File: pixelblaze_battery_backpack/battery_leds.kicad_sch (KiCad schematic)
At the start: 23 parts, among them J10 Conn_01x04, J11 Conn_01x04, J14 Conn_01x04, J15 Conn_01x04

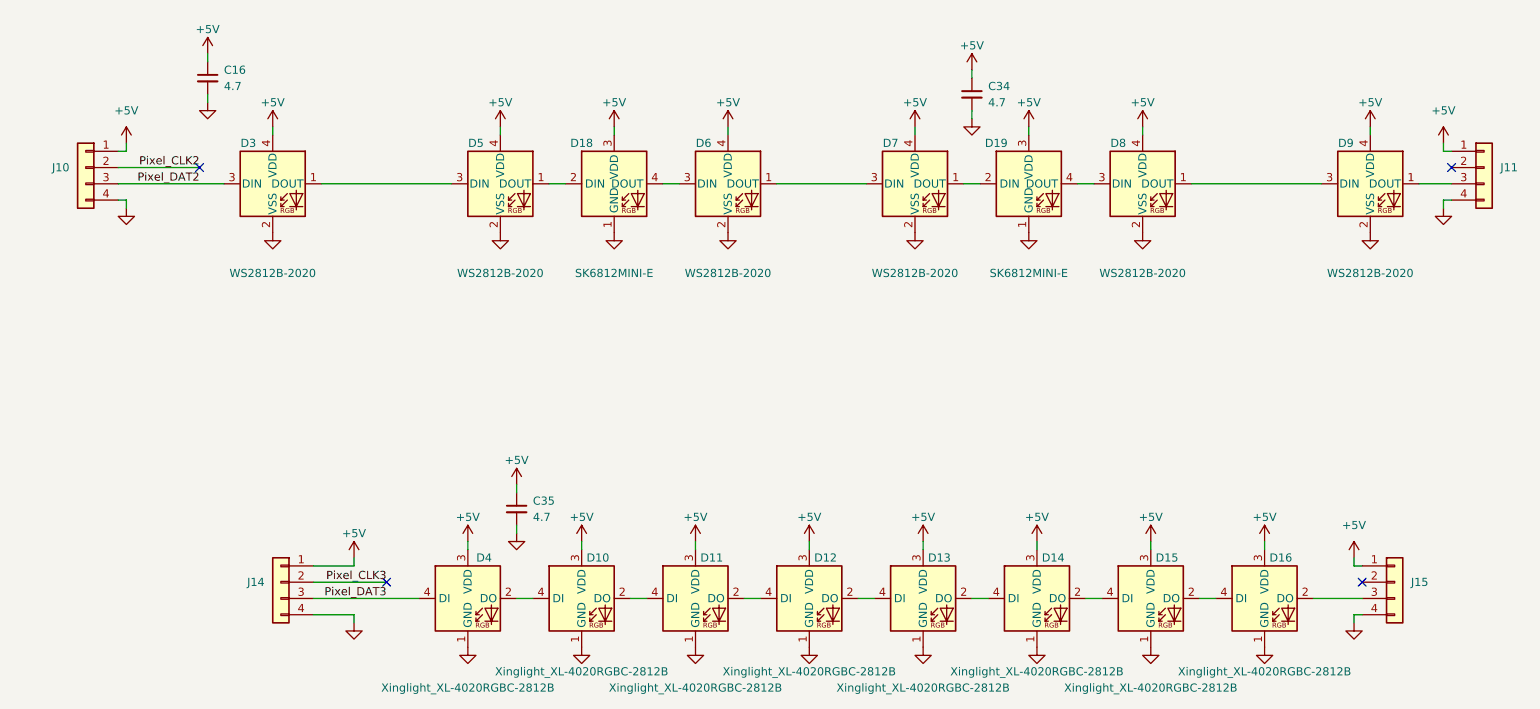
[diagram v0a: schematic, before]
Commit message: Finalized V2.
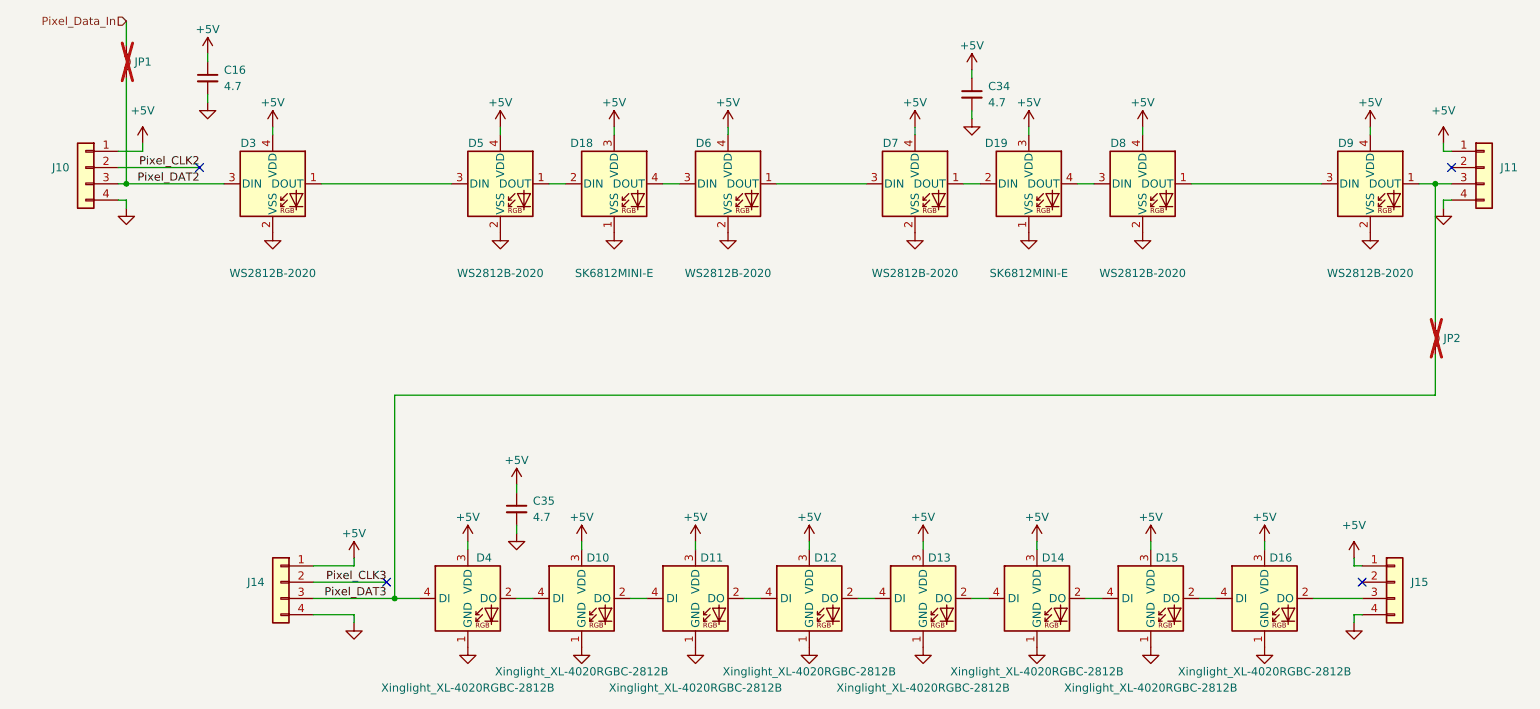
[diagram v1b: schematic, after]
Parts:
- added JP1, JP2: Jumper_2_Small_Bridged, Jumper:SolderJumper-2_P1.3mm_Bridged_RoundedPad1.0x1.5mm, symbol Jumper:Jumper_2_Small_Bridged
- D10, D11, D12, D13, D14, D15, D16, D4: FT Position Offset (none) -> 0,-0.75; FT Rotation Offset (none) -> 180; JLCPCB Part No. (none) -> C3647024; MPN (none) -> XL-4020RGBC-2812B
- D18, D19: JLCPCB Part No. (none) -> C5149201; MPN (none) -> SK6812MINI-E
- D3, D5, D6, D7, D8, D9: FT Rotation Offset (none) -> 180
- J10, J11, J14, J15: FT Position Offset (none) -> 0,-0.8125; FT Rotation Offset (none) -> 180; now in the parts list
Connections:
- net Pixel_DAT2: now also JP1.2 (B)
- net Pixel_DAT3: now also JP2.2 (B)
- net at D9.1 (DOUT), J11.3 (Pin_3): now also JP2.1 (A)
- new net Pixel_Data_In: JP1.1 (A)
